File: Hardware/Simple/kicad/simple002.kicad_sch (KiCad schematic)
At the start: 31 parts

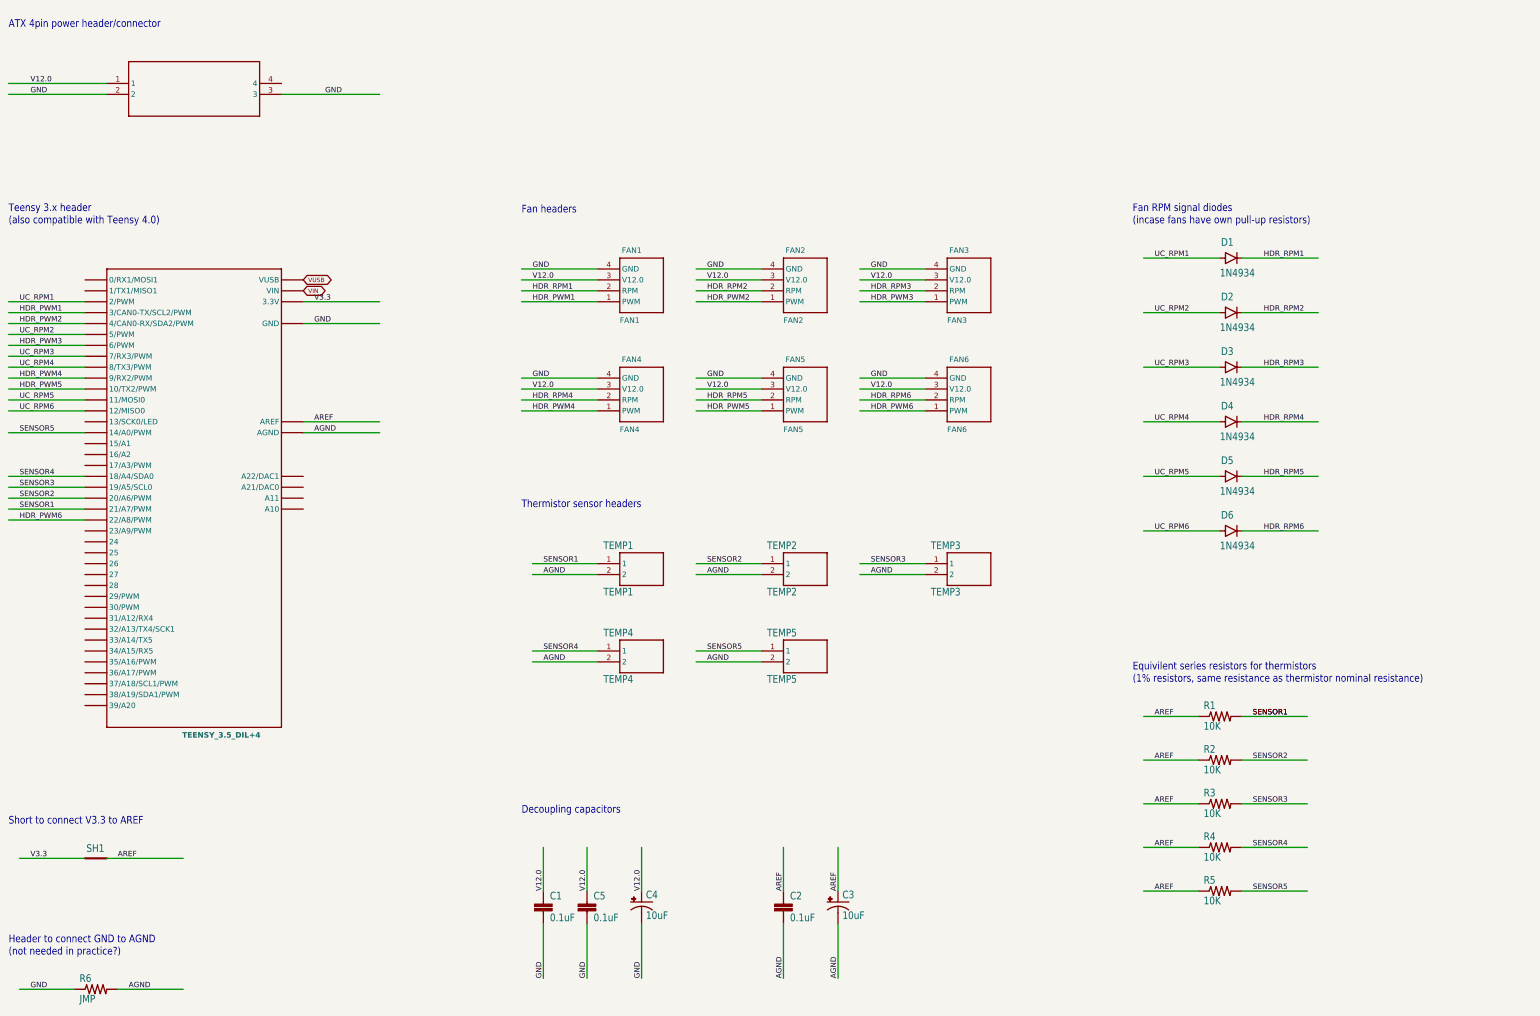
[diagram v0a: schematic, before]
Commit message: contd
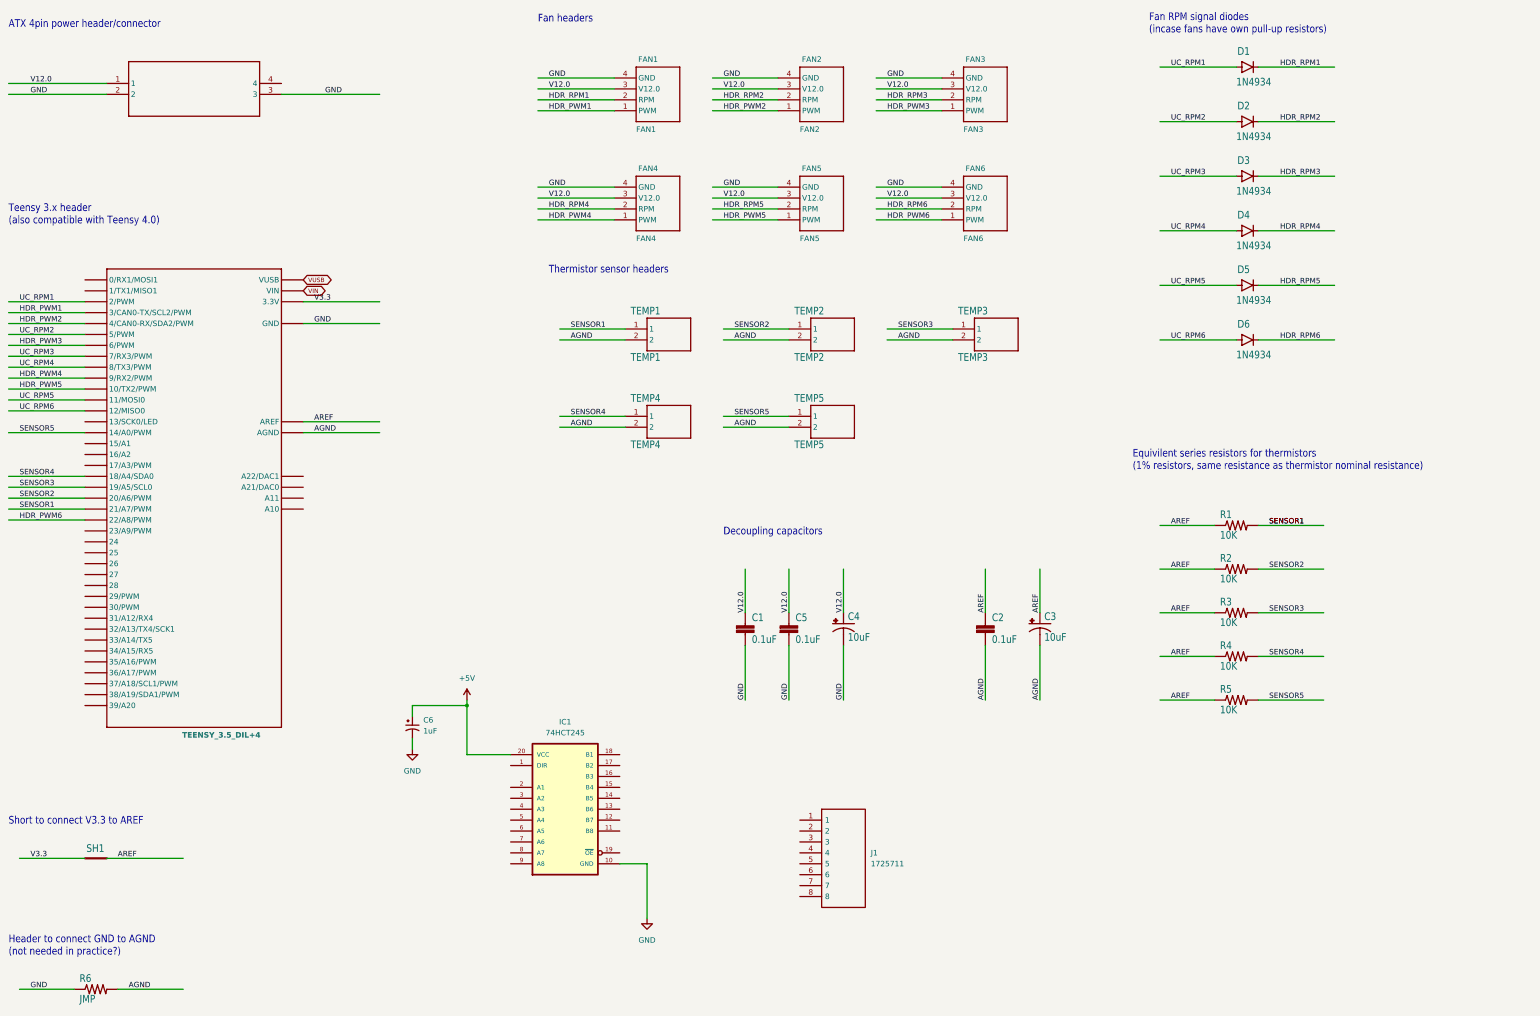
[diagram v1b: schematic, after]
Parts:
- added C6: 1uF, symbol Device:C_Polarized_Small_US
- added IC1: 74HCT245, symbol 74HCT245:74HCT245
- added J1: 1725711, 1725711, symbol 1725711:1725711
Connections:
- net GND: now also C6.2, IC1.10 (GND)
- new net +5V: C6.1, IC1.20 (VCC)
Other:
- moved on the sheet: C1, C2, C3, C4, C5, D1, D2, D3, D4, D5, D6, FAN1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
